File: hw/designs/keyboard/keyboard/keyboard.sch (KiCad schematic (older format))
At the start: 25 parts, among them J1 Conn_01x08_Female, Q1 2N2222A, Q2 2N2222A, Q3 2N2222A, Q4 2N2222A, Q5 2N2222A, Q6 2N2222A, Q7 2N2222A, Q8 2N2222A

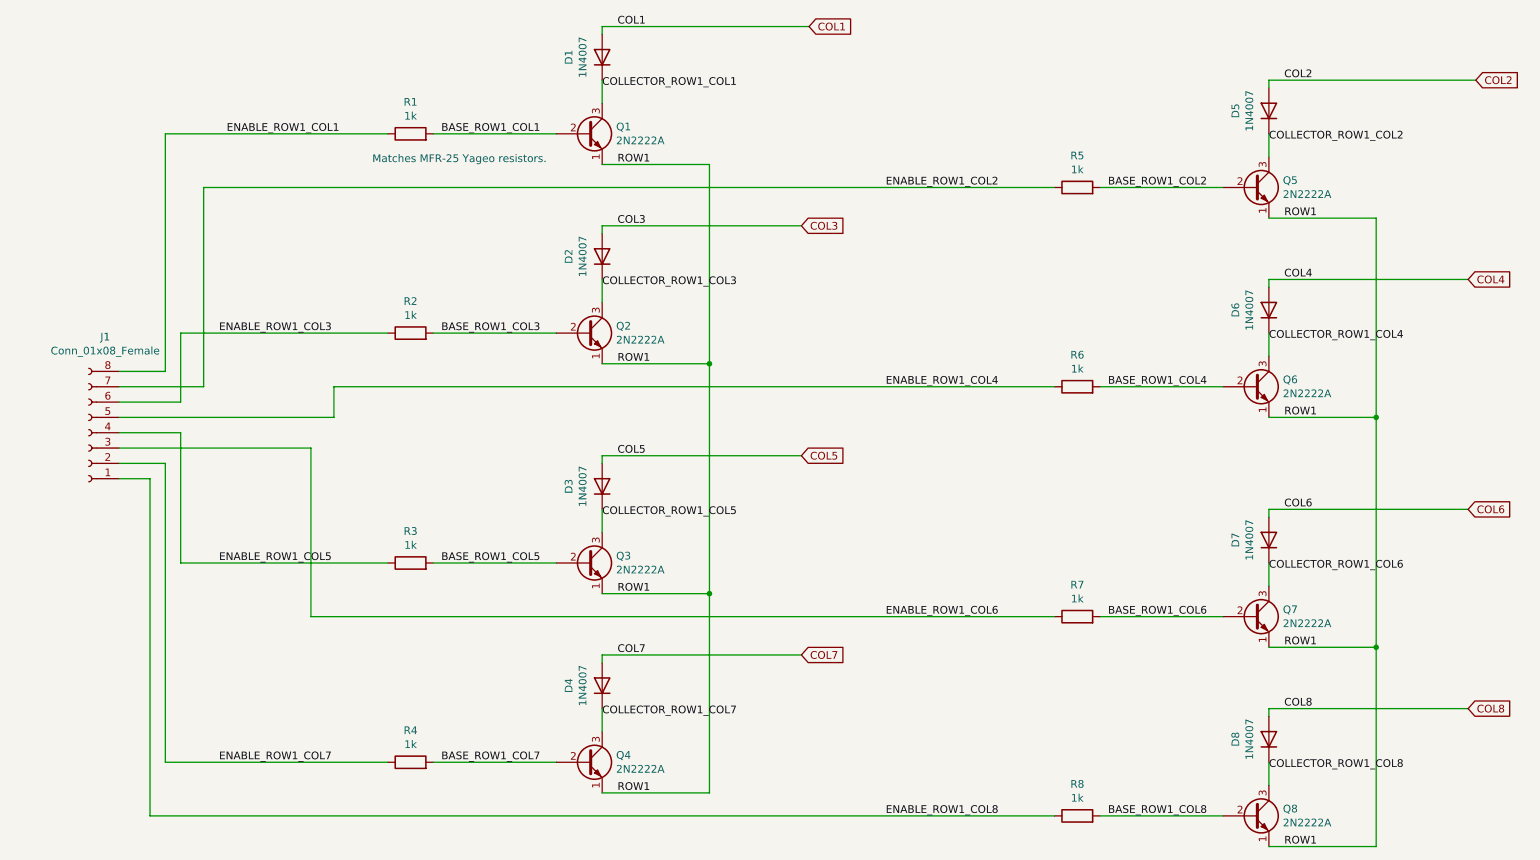
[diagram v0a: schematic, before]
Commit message: Adding sheets
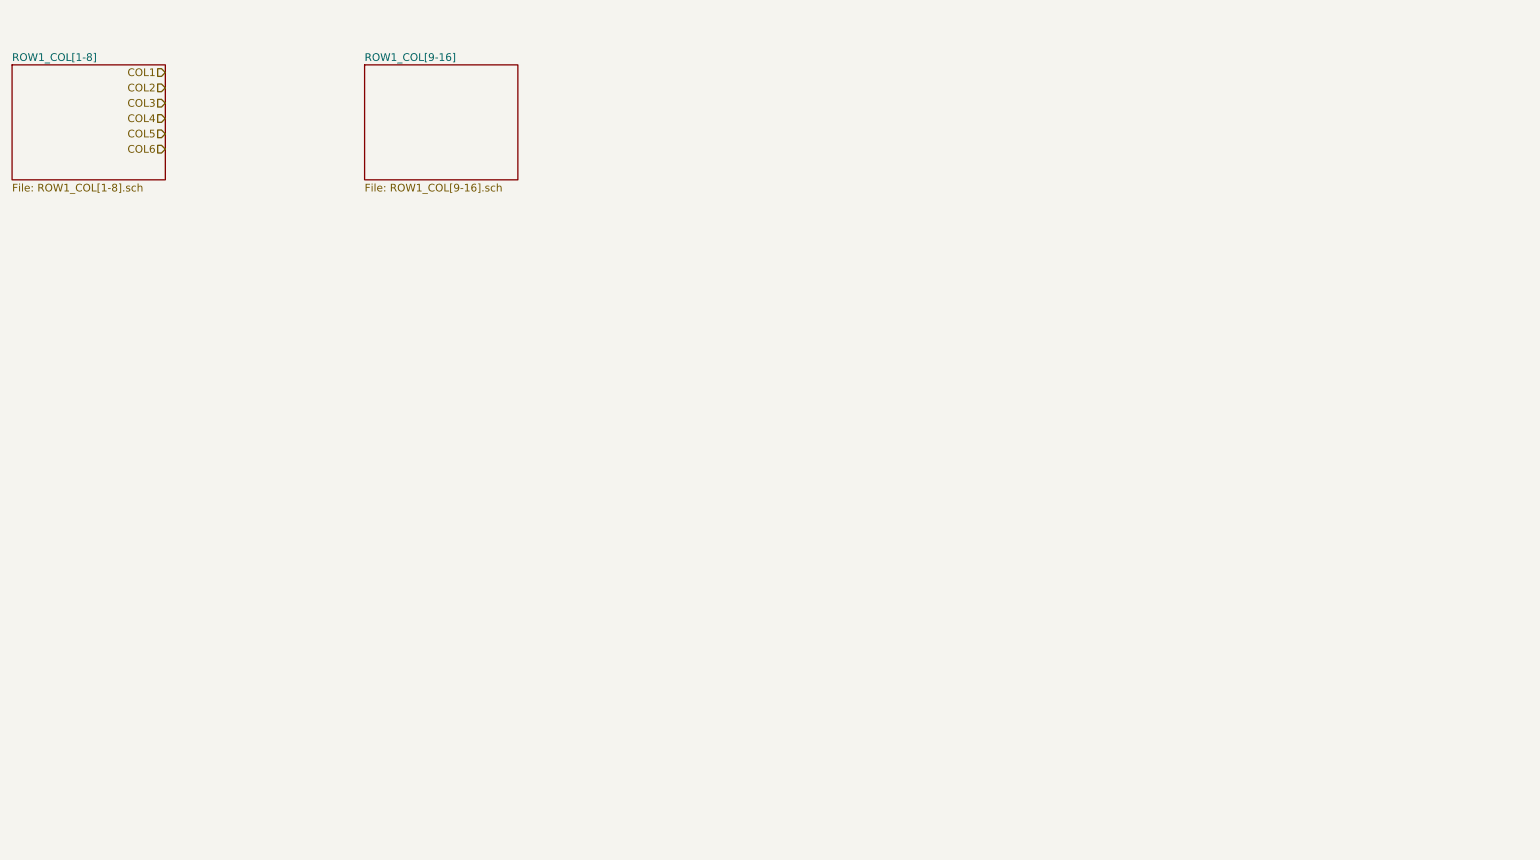
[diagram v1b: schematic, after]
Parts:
- removed D1, D2, D3, D4, D5, D6, D7, D8: 1N4007, Diode_THT:D_DO-41_SOD81_P10.16mm_Horizontal, symbol Diode:1N4007
- removed J1: Conn_01x08_Female, Connector_PinSocket_2.54mm:PinSocket_1x08_P2.54mm_Vertical, symbol Connector:Conn_01x08_Female
- removed Q1, Q2, Q3, Q4, Q5, Q6, Q7, Q8: 2N2222A, Package_TO_SOT_THT:TO-92_Inline, symbol Transistor_BJT:2N3904
- removed R1, R2, R3, R4, R5, R6, R7, R8: 1k, Resistor_THT:R_Axial_DIN0207_L6.3mm_D2.5mm_P10.16mm_Horizontal, symbol Device:R
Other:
- note removed: "Matches MFR-25 Yageo resistors."
